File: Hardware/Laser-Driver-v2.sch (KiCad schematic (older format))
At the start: 36 parts

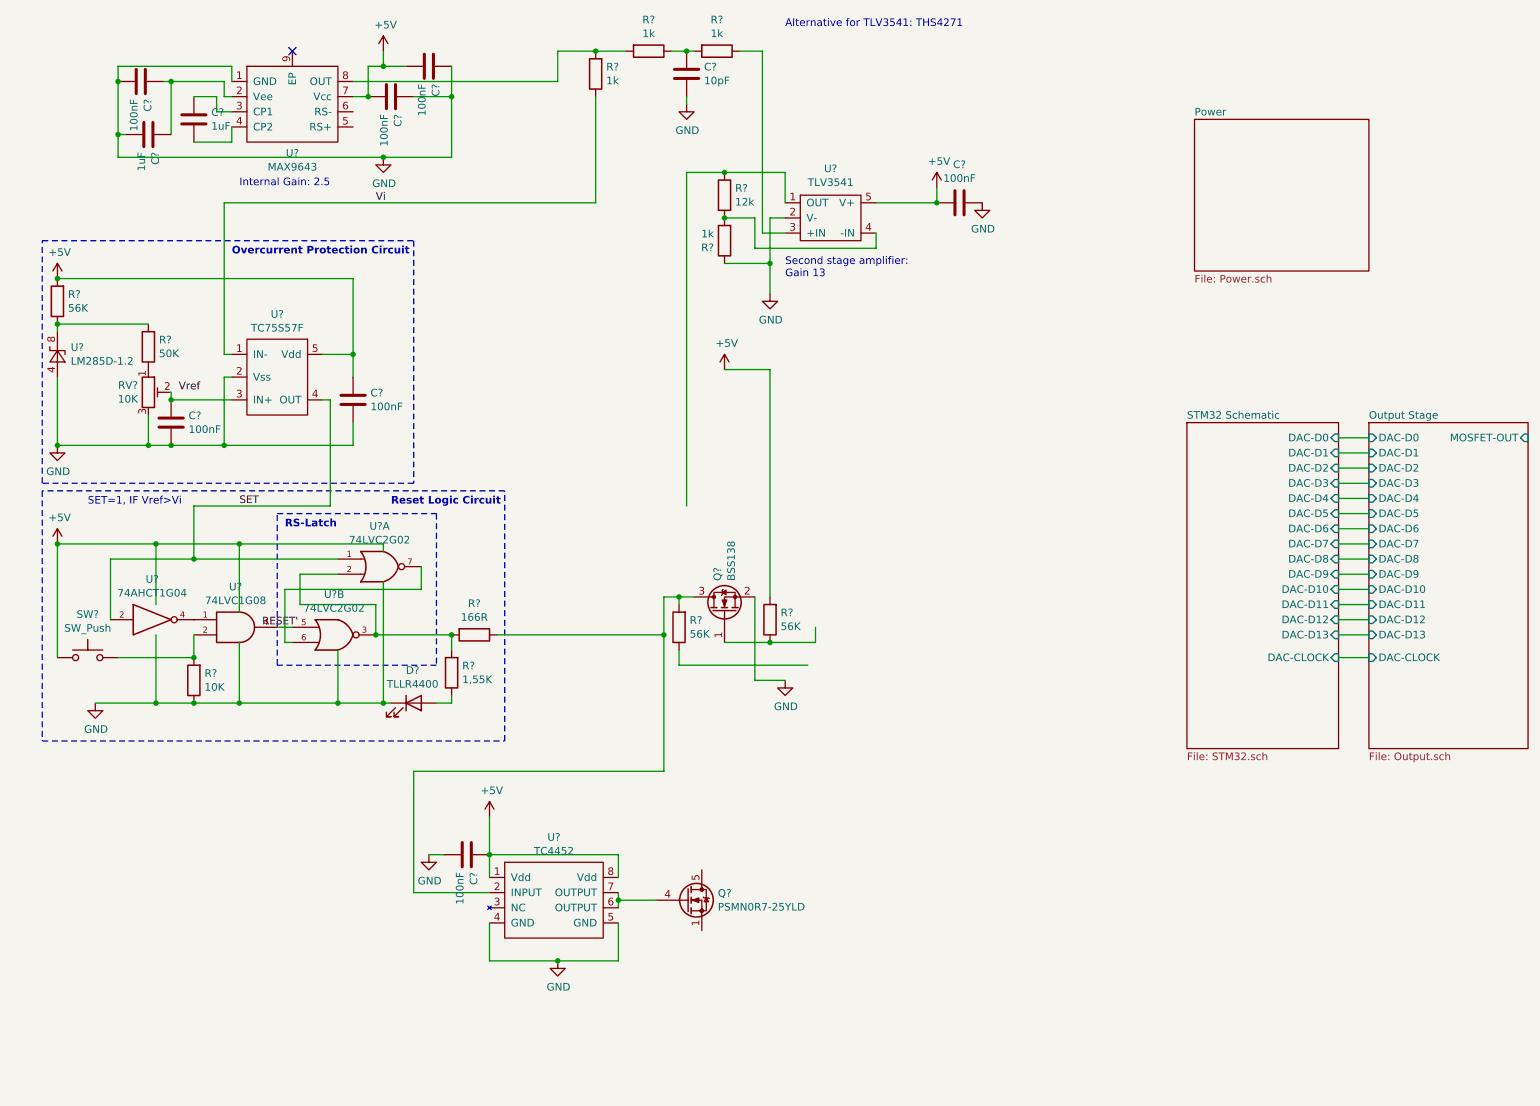
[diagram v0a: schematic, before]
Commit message: added dissipation Mosfet, cleaned up Main sheet
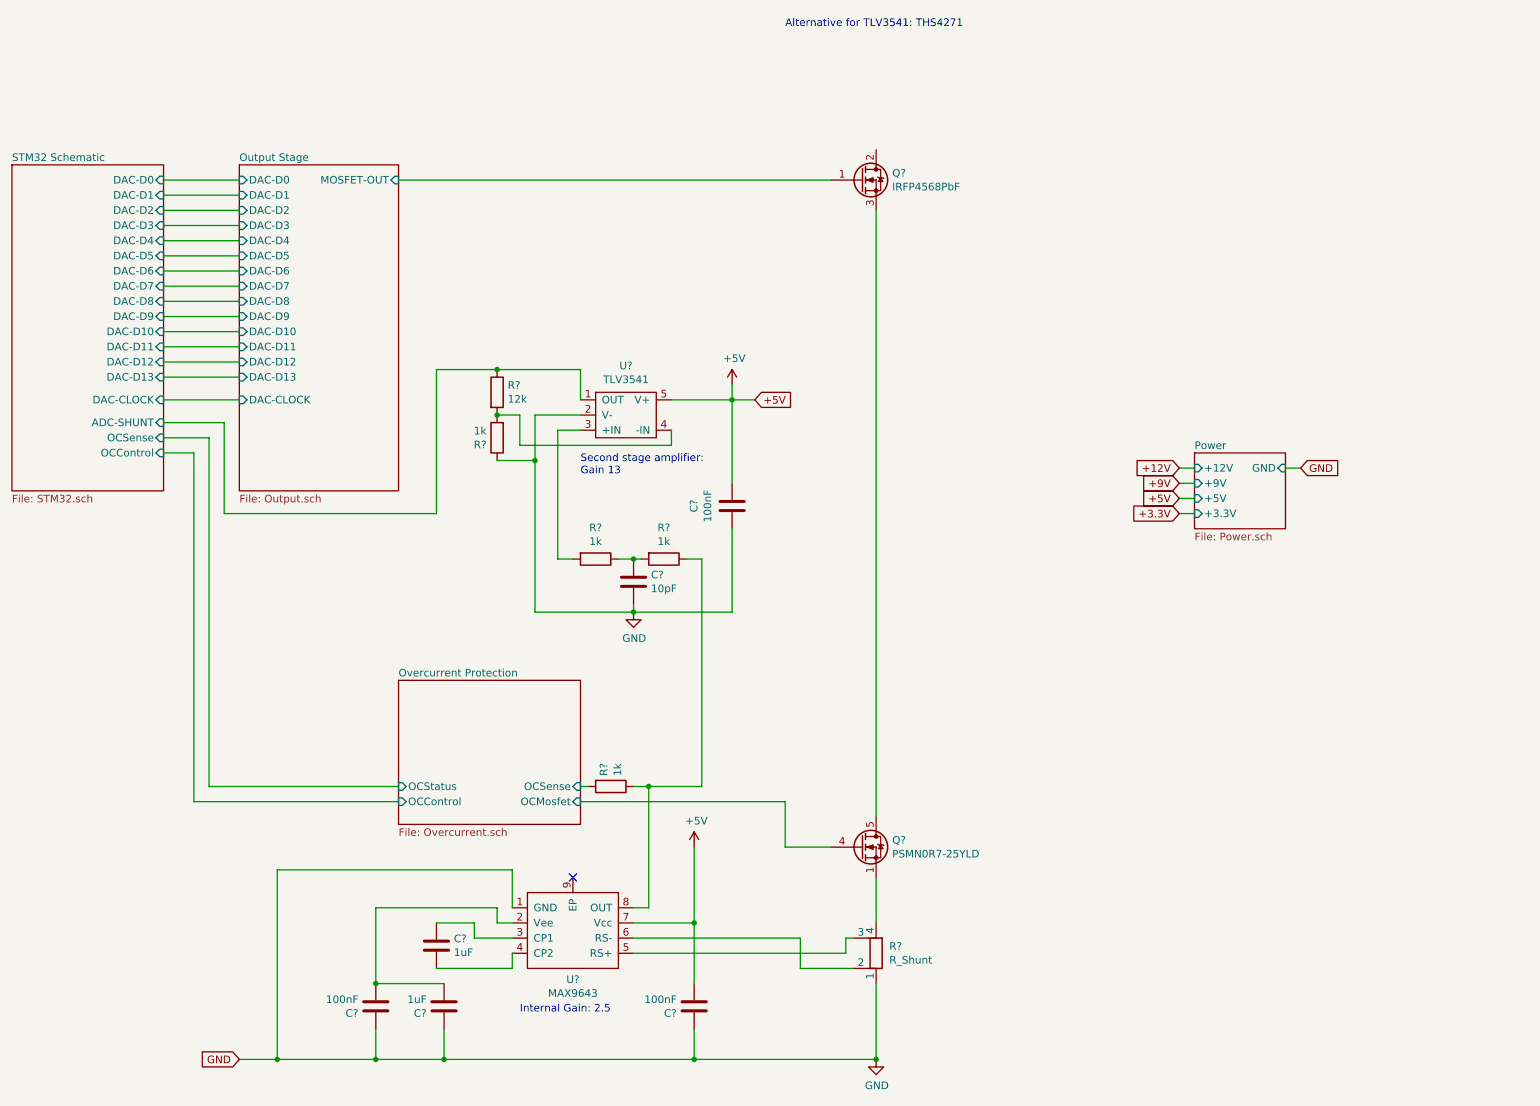
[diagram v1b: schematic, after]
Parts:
- removed C? (x4): 100nF, symbol Device:C
- removed D?: TLLR4400, symbol Device:LED
- removed Q?: BSS138, Package_TO_SOT_SMD:SOT-23, symbol Transistor_FET:BSS138
- removed R? (x3): 56K, symbol Device:R
- removed R?: 50K, symbol Device:R
- removed R?: 10K, symbol Device:R
- removed R?: 166R, symbol Device:R
- removed R?: 1,55K, symbol Device:R
- removed RV?: 10K, symbol Device:R_POT_TRIM
- removed SW?: SW_Push, symbol Switch:SW_Push
- removed U?: TC75S57F, symbol OS-LD:TC75S57F
- removed U?: TC4452, Package_SO:SOIC-8_3.9x4.9mm_P1.27mm, symbol OS-LD:TC4452
- removed U?: LM285D-1.2, Package_SO:SOIC-8_3.9x4.9mm_P1.27mm, symbol Reference_Voltage:LM285D-1.2
- removed U? (x2): 74LVC2G02, symbol 74xGxx:74LVC2G02
- removed U?: 74LVC1G08, symbol 74xGxx:74LVC1G08
- removed U?: 74AHCT1G04, symbol 74xGxx:74AHCT1G04
- added Q?: IRFP4568PbF, Package_TO_SOT_THT:TO-247-3_Vertical, symbol OS-LD:IRFP4568PbF
- added R?: R_Shunt, symbol Device:R_Shunt
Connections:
- net Vi is gone; now on an unnamed net: R?.1
- net +5V: now also C?.1; no longer C?.2
- net GND: now also C?.1, C?.1, C?.2, R?.1; no longer C?.1, C?.2, C?.2
- net Output Stage/MOSFET-OUT: now also Q?.1 (G)
- net at U?.5 (RS+): now also R?.3
- net at U?.6 (RS-): now also R?.2
- net STM32 Schematic/ADC-SHUNT: now reaches R?.1, U?.1 (OUT)
- net at R?.1: now also U?.8 (OUT); no longer U?.3 (+IN)
- net at Q?.1 (S), Q?.2 (S), Q?.3 (S): now also R?.4
- net Overcurrent Protection/OCMosfet: now reaches Q?.4 (G)
- net at Q?.5 (D): now also Q?.3 (S)
- new net: C?.2, C?.2, U?.2 (Vee)
- new net: R?.2, U?.3 (+IN)
- new net Overcurrent Protection/OCSense: R?.2
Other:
- note removed: "Overcurrent Protection Circuit"
- note removed: "RS-Latch"
- note removed: "Reset Logic Circuit"
- note removed: "SET=1, IF Vref>Vi"
- moved on the sheet: C?, Q?, R?, U?

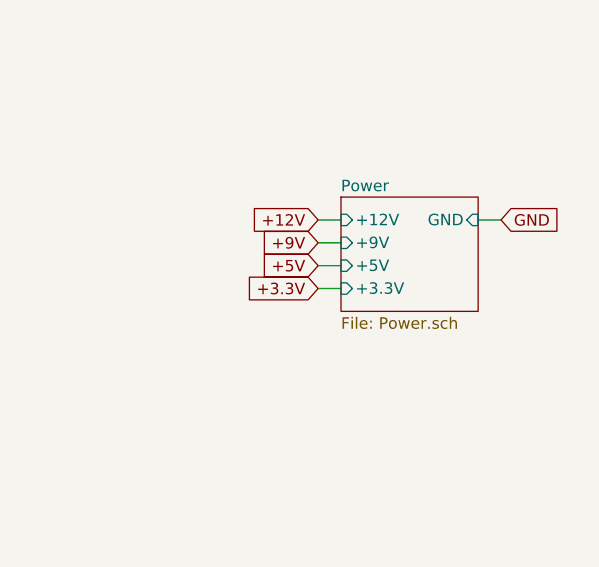
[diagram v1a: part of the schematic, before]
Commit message: cleaned up power supplies
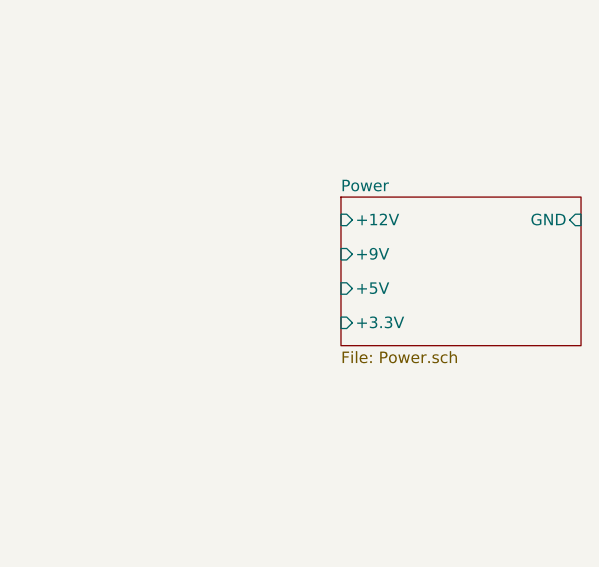
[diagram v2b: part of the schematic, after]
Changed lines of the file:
@@
 	1750 3000 2250 3000
 $Sheet
-S 8550 3350 600  500
+S 8550 3350 1050 650
 U 5D12441E
 F0 "Power" 50
 F1 "Power.sch" 50
 F2 "+12V" I L 8550 3450 50
-F3 "GND" I R 9150 3450 50
-F4 "+5V" I L 8550 3650 50
-F5 "+3.3V" I L 8550 3750 50
-F6 "+9V" I L 8550 3550 50
+F3 "GND" I R 9600 3450 50
+F4 "+5V" I L 8550 3750 50
+F5 "+3.3V" I L 8550 3900 50
+F6 "+9V" I L 8550 3600 50
 $EndSheet
 Text Notes 4100 7050 0    50   ~ 0
@@
 Wire Wire Line
 	1950 3350 1750 3350
-Text GLabel 8450 3450 0    50   Input ~ 0
-+12V
-Text GLabel 8450 3550 0    50   Input ~ 0
-+9V
-Text GLabel 8450 3650 0    50   Input ~ 0
-+5V
-Text GLabel 8450 3750 0    50   Input ~ 0
-+3.3V
-Text GLabel 9250 3450 2    50   Input ~ 0
-GND
-Wire Wire Line
-	8450 3450 8550 3450
-Wire Wire Line
-	8450 3550 8550 3550
-Wire Wire Line
-	8450 3650 8550 3650
-Wire Wire Line
-	8450 3750 8550 3750
 Connection ~ 5500 3000
 Wire Wire Line
 	5500 3000 5500 2900
-Wire Wire Line
-	9150 3450 9250 3450
 $Comp
 L power:+5V #PWR?
